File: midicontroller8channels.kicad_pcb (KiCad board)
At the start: 2 copper layers, 60 x 80 mm, 31 parts, among them J1 Conn_01x02_Male, J10 Conn_01x02_Male, J11 Conn_01x02_Male, J12 Conn_01x02_Male, J13 Conn_01x12_Male, J14 Conn_01x12_Male, J15 Conn_01x12_Male, J16 Conn_01x12_Male, J17 Conn_01x05_Male, J18 Conn_01x06_Male, J19 Conn_01x04_Male, J2 Conn_01x02_Male, J3 Conn_01x02_Male, J4 Conn_01x02_Male, J5 Conn_01x12_Male, J6 Conn_01x12_Male, J7 Conn_01x12_Male, J8 Conn_01x12_Male, J9 Conn_01x02_Male, U1 4051, U2 4051, U3 4051, U4 4051

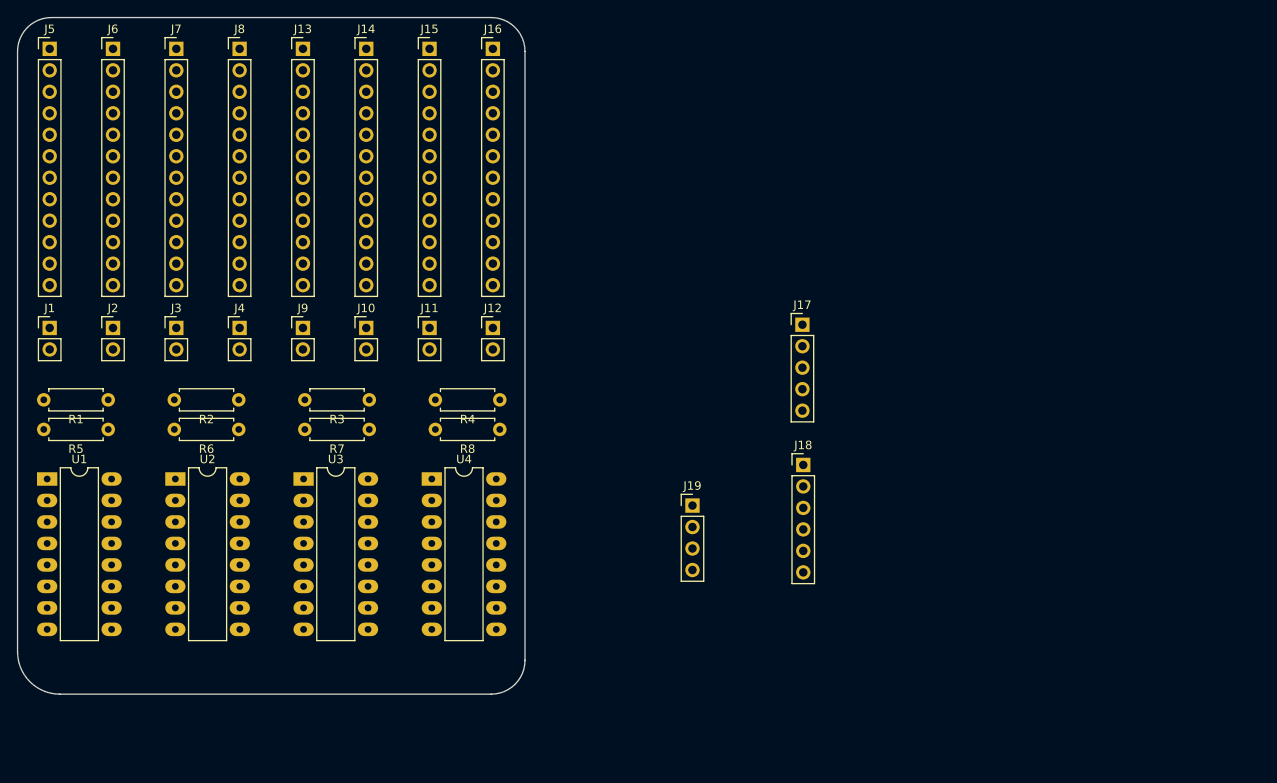
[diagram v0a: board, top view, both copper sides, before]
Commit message: finalizado
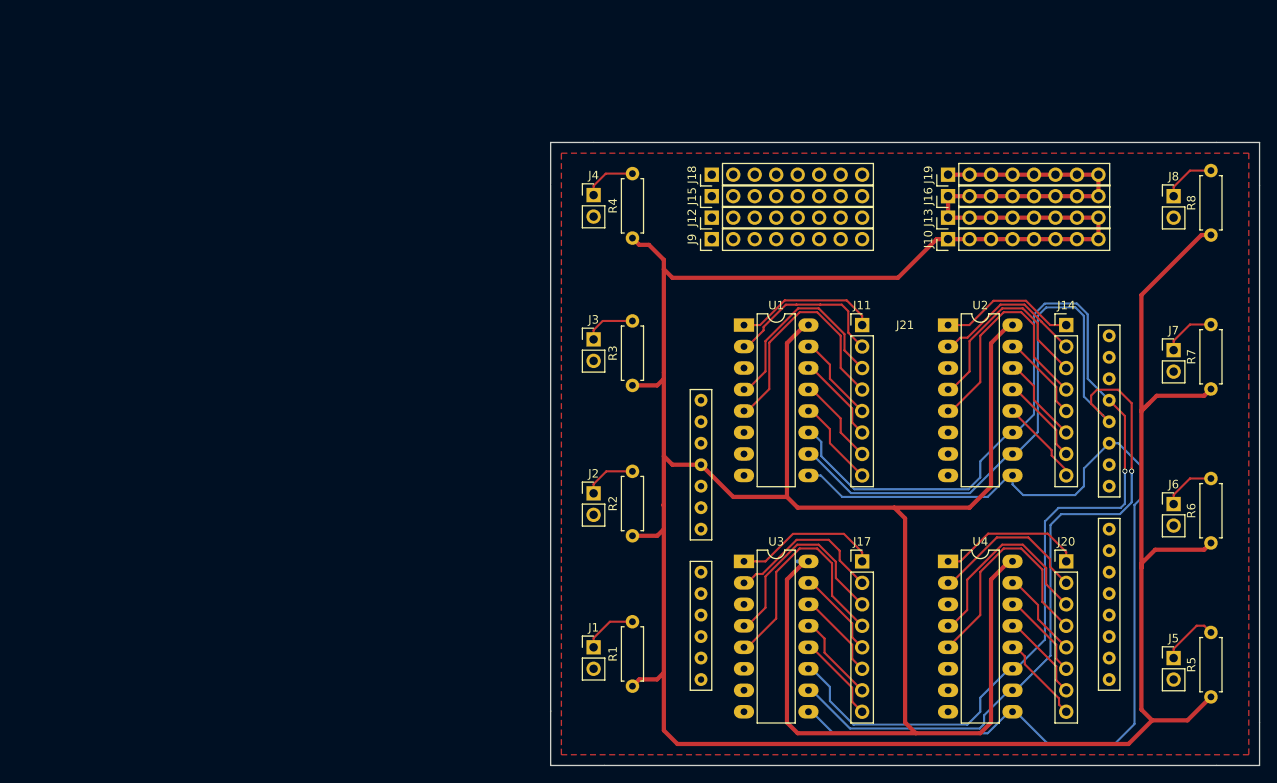
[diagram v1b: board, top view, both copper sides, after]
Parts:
- added J20: Conn_01x08_Male, Pin_Headers:Pin_Header_Straight_1x08_Pitch2.54mm, F.Cu at (174.0, 114.3)
- added J21: arduinoUnoPinout, arduino:arduinoUnoPinout, F.Cu at (154.9, 109.2)
- J10, J11, J12, J9: value Conn_01x02_Male -> Conn_01x08_Male; footprint Pin_Headers:Pin_Header_Straight_1x02_Pitch2.54mm -> Pin_Headers:Pin_Header_Straight_1x08_Pitch2.54mm
- J13, J14, J15, J16: value Conn_01x12_Male -> Conn_01x08_Male; footprint Pin_Headers:Pin_Header_Straight_1x12_Pitch2.54mm -> Pin_Headers:Pin_Header_Straight_1x08_Pitch2.54mm
- J17: value Conn_01x05_Male -> Conn_01x08_Male; footprint Pin_Headers:Pin_Header_Straight_1x05_Pitch2.54mm -> Pin_Headers:Pin_Header_Straight_1x08_Pitch2.54mm
- J18: value Conn_01x06_Male -> Conn_01x08_Male; footprint Pin_Headers:Pin_Header_Straight_1x06_Pitch2.54mm -> Pin_Headers:Pin_Header_Straight_1x08_Pitch2.54mm
- J19: value Conn_01x04_Male -> Conn_01x08_Male; footprint Pin_Headers:Pin_Header_Straight_1x04_Pitch2.54mm -> Pin_Headers:Pin_Header_Straight_1x08_Pitch2.54mm
- J5, J6, J7, J8: value Conn_01x12_Male -> Conn_01x02_Male; footprint Pin_Headers:Pin_Header_Straight_1x12_Pitch2.54mm -> Pin_Headers:Pin_Header_Straight_1x02_Pitch2.54mm
- moved J5 151.2 mm to (186.7, 125.7)
- moved J6 136.5 mm to (186.7, 107.5)
- moved R5 134.2 mm to (191.1, 130.3), turned to 90 degrees
- moved J7 123.2 mm to (186.7, 89.3)
- moved R6 115.7 mm to (191.1, 112.1), turned to 90 degrees
- moved J8 111.8 mm to (186.7, 71.1)
- moved R7 99.6 mm to (191.1, 93.9), turned to 90 degrees
- moved U2 93.2 mm to (160.0, 86.4)
- moved J14 89.0 mm to (174.0, 86.4)
- moved R8 87.2 mm to (191.1, 75.7), turned to 90 degrees
- moved U1 84.4 mm to (135.9, 86.4)
- moved J13 78.8 mm to (160.0, 73.7), turned to 90 degrees
- moved J1 74.6 mm to (118.1, 124.5)
- moved R1 70.6 mm to (122.7, 129.1), turned to 90 degrees
- moved J10 69.6 mm to (160.0, 76.2), turned to 90 degrees
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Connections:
- J10 pad 1: D7 -> +5V
- J10 pad 2: GND -> +5V
- J11 pad 1: D8 -> P0_0
- J11 pad 2: GND -> P1_0
- J12 pad 1: D9 -> GND
- J13 pad 2: P4_0 -> +5V
- J13 pad 3: GND -> +5V
- J13 pad 5: P4_1 -> +5V
- J13 pad 6: GND -> +5V
- J13 pad 8: P4_2 -> +5V
- J14 pad 1: +5V -> P0_1
- J14 pad 2: P5_0 -> P1_1
- J14 pad 3: GND -> P2_1
- J14 pad 4: +5V -> P3_1
- J14 pad 5: P5_1 -> P4_1
- J14 pad 6: GND -> P5_1
- J14 pad 7: +5V -> P6_1
- J14 pad 8: P5_2 -> P7_1
- J15 pad 1: +5V -> GND
- J15 pad 2: P6_0 -> GND
- J15 pad 4: +5V -> GND
- J15 pad 5: P6_1 -> GND
- J15 pad 7: +5V -> GND
- J15 pad 8: P6_2 -> GND
- J16 pad 2: P7_0 -> +5V
- J16 pad 3: GND -> +5V
- J16 pad 5: P7_1 -> +5V
- J16 pad 6: GND -> +5V
- J16 pad 8: P7_2 -> +5V
- J17 pad 1: D12 -> P0_2
- J17 pad 2: D11 -> P1_2
- J17 pad 3: D10 -> P2_2
- J17 pad 4: D9 -> P3_2
- J17 pad 5: D8 -> P4_2
- J18 pad 1: D7 -> GND
- J18 pad 2: D6 -> GND
- J18 pad 3: D5 -> GND
- J18 pad 4: D4 -> GND
- J18 pad 5: D3 -> GND
- J18 pad 6: D2 -> GND
- J19 pad 1: A0 -> +5V
- J19 pad 2: A1 -> +5V
- J19 pad 3: A2 -> +5V
- J19 pad 4: A3 -> +5V
- J5 pad 1: +5V -> D6
- J5 pad 2: P0_0 -> GND
- J6 pad 1: +5V -> D7
- J6 pad 2: P1_0 -> GND
- J7 pad 1: +5V -> D8
- J7 pad 2: P2_0 -> GND
- J8 pad 1: +5V -> D9
- J8 pad 2: P3_0 -> GND
- J9 pad 1: D6 -> GND
- U1 pad 1: P4_0 -> P0_0
- U1 pad 12: P3_0 -> P7_0
- U1 pad 13: P0_0 -> P6_0
- U1 pad 14: P1_0 -> P5_0
- U1 pad 15: P2_0 -> P4_0
- U1 pad 2: P6_0 -> P1_0
- U1 pad 4: P7_0 -> P2_0
- U1 pad 5: P5_0 -> P3_0
- U2 pad 1: P4_1 -> P0_1
- U2 pad 12: P3_1 -> P7_1
- U2 pad 13: P0_1 -> P6_1
- U2 pad 14: P1_1 -> P5_1
- U2 pad 15: P2_1 -> P4_1
- U2 pad 2: P6_1 -> P1_1
- U2 pad 4: P7_1 -> P2_1
- U2 pad 5: P5_1 -> P3_1
- U3 pad 1: P4_2 -> P0_2
- U3 pad 12: P3_2 -> P7_2
- U3 pad 13: P0_2 -> P6_2
- U3 pad 14: P1_2 -> P5_2
- U3 pad 15: P2_2 -> P4_2
- U3 pad 2: P6_2 -> P1_2
- U3 pad 4: P7_2 -> P2_2
- U3 pad 5: P5_2 -> P3_2
- U4 pad 1: P4_3 -> P0_3
- U4 pad 12: P3_3 -> P7_3
- U4 pad 13: P0_3 -> P6_3
- U4 pad 14: P1_3 -> P5_3
- U4 pad 15: P2_3 -> P4_3
- U4 pad 2: P6_3 -> P1_3
- U4 pad 4: P7_3 -> P2_3
- U4 pad 5: P5_3 -> P3_3
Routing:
- net +5V: track 0.00 -> 516.9 mm
- net D11: track 0.00 -> 148.1 mm, vias 0 -> 1
- net D12: track 0.00 -> 139.8 mm, vias 0 -> 1
- net D10: track 0.00 -> 121.9 mm
- net P3_2: track 0.00 -> 28.1 mm
- net P3_0: track 0.00 -> 28.1 mm
- net P3_1: track 0.00 -> 28.1 mm
- net P3_3: track 0.00 -> 27.8 mm
- net P2_2: track 0.00 -> 24.2 mm
- net P2_3: track 0.00 -> 24.1 mm
- net P2_0: track 0.00 -> 24.1 mm
- net P2_1: track 0.00 -> 24.1 mm
- net P1_0: track 0.00 -> 19.8 mm
- net P1_3: track 0.00 -> 18.9 mm
- net P1_2: track 0.00 -> 18.9 mm
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- added copper zone on F.Cu, net GND
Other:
- board size 60 x 80 mm -> 83.8 x 73.7 mm
- net class alimentacion: clearance 0.4 -> 0.6
